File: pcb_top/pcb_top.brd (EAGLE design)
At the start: 32 x 37.3 mm, 6 parts, among them X1 FH12-14S-0.5SH

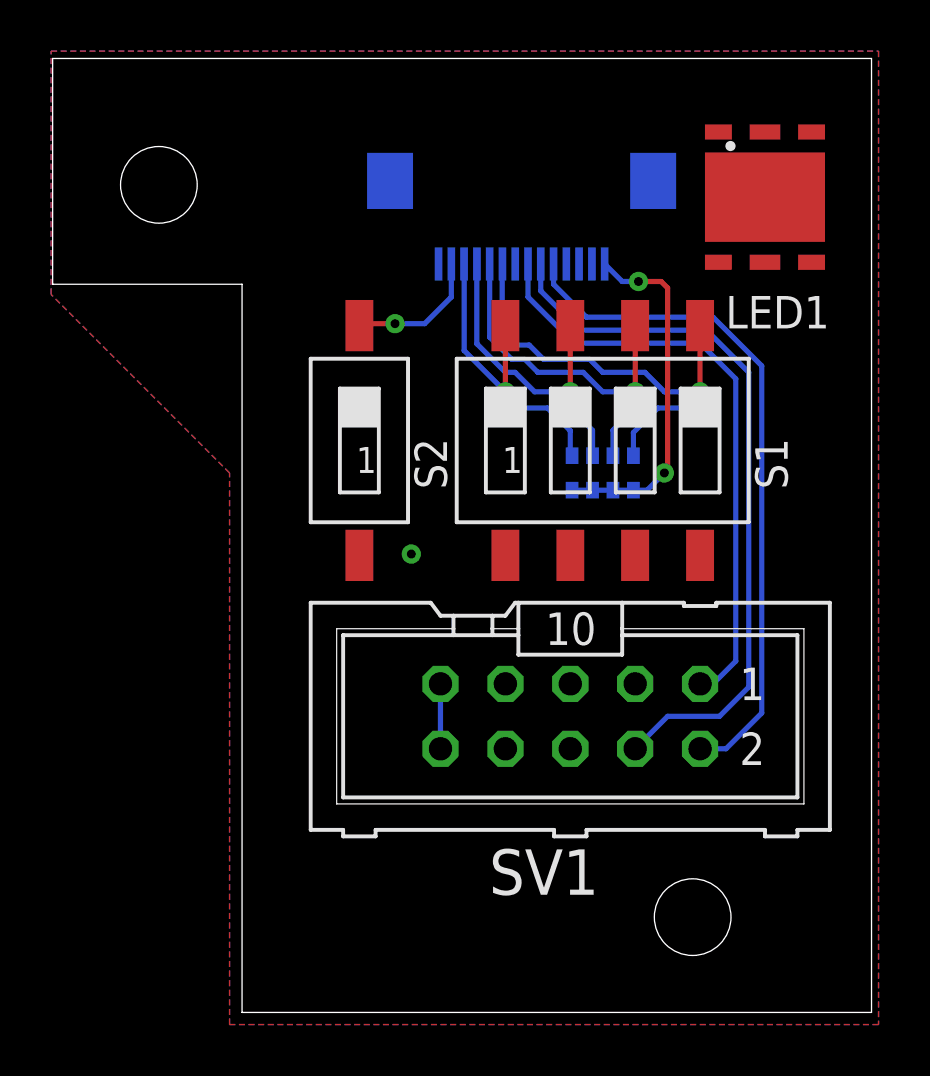
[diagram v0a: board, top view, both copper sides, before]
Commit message: finished v1.0
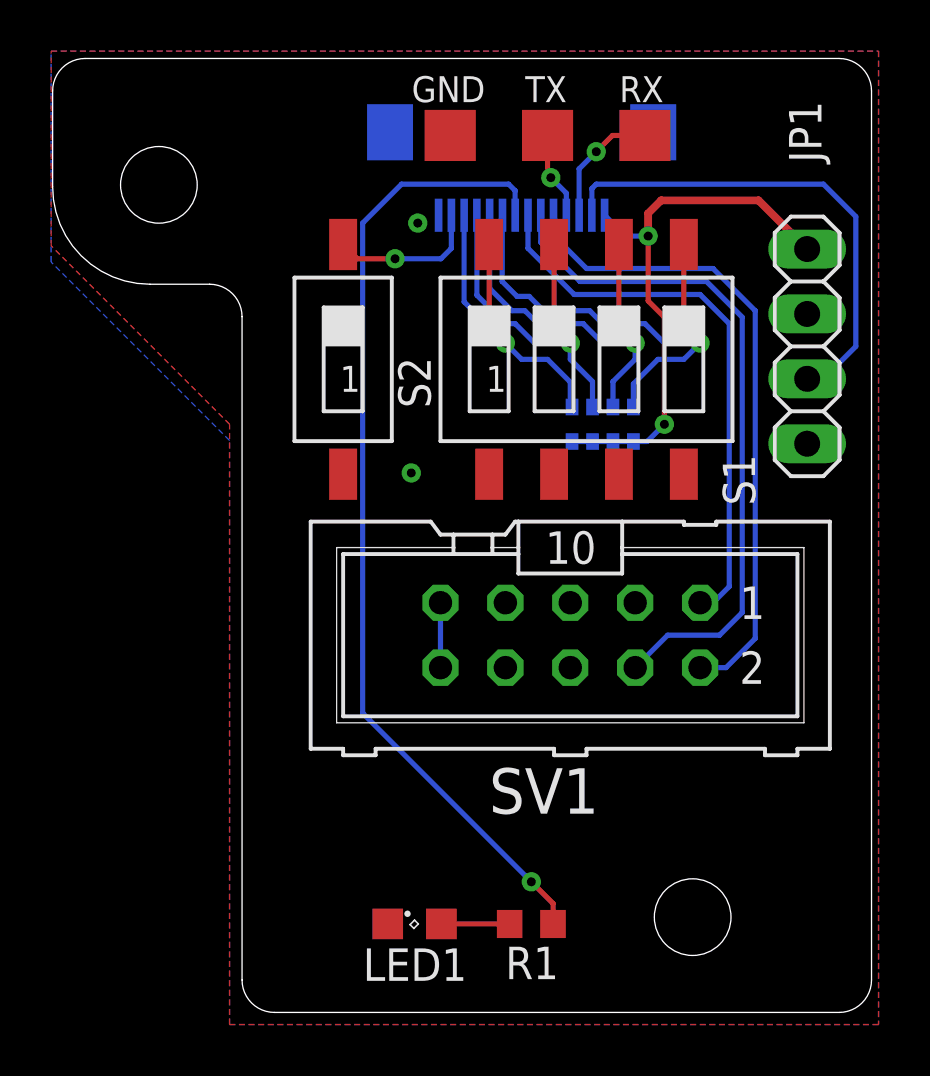
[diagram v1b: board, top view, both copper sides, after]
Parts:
- added GND, RX, TX: TPTP20SQ, testpad:TP20SQ
- added JP1: (no value), pinhead:1X04
- added R1: (no value), rcl:R0603
- LED1: value F50360 -> (none); device led:F50360 -> led:SML0805
- moved LED1 31.6 mm to (-17.9, 3.43), turned to 0 degrees
- moved S1 3.24 mm to (-11.2, 25.5)
- moved S2 3.24 mm to (-20.7, 25.5)
- moved SV1 3.17 mm to (-11.8, 14.7)
- moved X1 1.91 mm to (-13.7, 34.4)
- moved RN1 1.90 mm to (-10.5, 23.0)
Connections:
- new net N$1: LED1.A, R1.1
- net 3,3V: now also JP1.1
- net GND: now also GND.TP, JP1.2, LED1.C
- net LED: now also R1.2
- net RX: now also RX.TP
- net STARTER: now also JP1.3
- net TX: now also TX.TP
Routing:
- net LED: track 0.00 -> 38.2 mm, vias 0 -> 1
- net STARTER: track 0.00 -> 19.5 mm
- net 3,3V: track 14.0 -> 21.7 mm
- net RX: track 0.00 -> 4.93 mm, vias 0 -> 1
- net TX: track 0.00 -> 3.43 mm, vias 0 -> 1
- net N$1: track 0.00 -> 2.67 mm
- net SW4: track 18.1 -> 19.6 mm
- net SW3: track 14.9 -> 16.4 mm
- net SW2: track 13.7 -> 15.2 mm
- net SW1: track 12.4 -> 14.0 mm
- net SWDIO: track 28.3 -> 26.8 mm
- net SWCLK: track 26.8 -> 25.4 mm
- net RST: track 23.6 -> 22.1 mm
- net ROBOT_ON: track 5.36 -> 5.93 mm
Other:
- outline, holes or cut-outs redrawn
- board text added: "Miras V1.0 minisumo Dominik Pluta Kamil Winnicki"

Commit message: minor changes
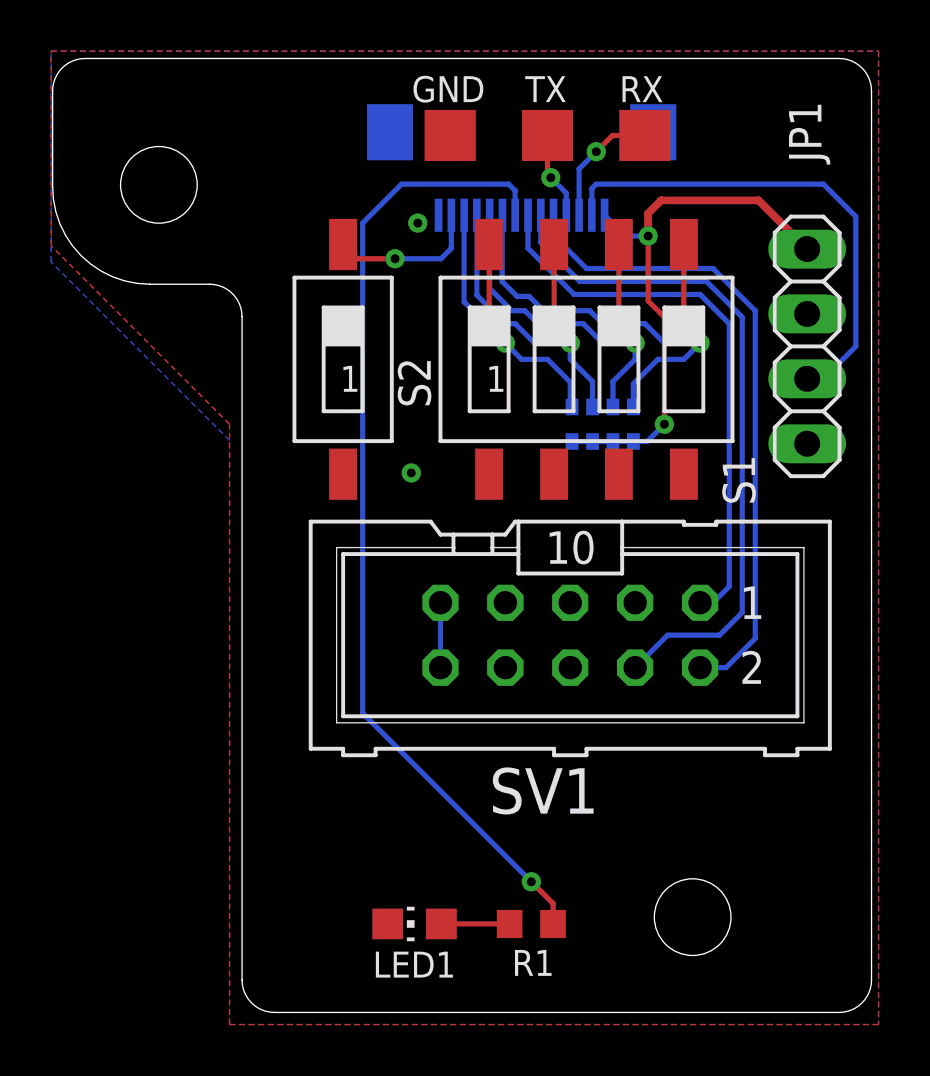
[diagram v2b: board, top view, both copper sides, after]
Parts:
- LED1: device led:SML0805 -> led:CHIP-LED0805
- turned LED1 to 90 degrees
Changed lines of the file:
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@@
 <attribute name="POPULARITY" value="9" x="-20.701" y="25.527" size="1.778" layer="27" display="off"/>
 </element>
-<element name="LED1" library="led" library_urn="urn:adsk.eagle:library:259" package="SML0805" package3d_urn="urn:adsk.eagle:package:15830/1" value="" x="-17.907" y="3.429" smashed="yes">
-<attribute name="NAME" x="-19.924" y="1.203" size="1.27" layer="25"/>
-<attribute name="POPULARITY" value="17" x="-17.907" y="3.429" size="1.778" layer="27" display="off"/>
-<attribute name="VALUE" x="-23.077" y="6.004" size="1.27" layer="27" rot="R270"/>
+<element name="LED1" library="led" library_urn="urn:adsk.eagle:library:259" package="CHIP-LED0805" package3d_urn="urn:adsk.eagle:package:15818/2" value="" x="-17.907" y="3.429" smashed="yes" rot="R90">
+<attribute name="NAME" x="-19.543" y="1.33" size="1.016" layer="25"/>
+<attribute name="POPULARITY" value="68" x="-17.907" y="3.429" size="1.778" layer="27" rot="R90" display="off"/>
+<attribute name="VALUE" x="-20.482" y="-1.741" size="1.27" layer="27"/>
 </element>
 <element name="X1" library="con-hirose" library_urn="urn:adsk.eagle:library:152" package="FH12-14S-0.5SH" package3d_urn="urn:adsk.eagle:package:7327/1" override_package3d_urn="urn:adsk.eagle:package:39279061/2" override_package_urn="urn:adsk.eagle:footprint:7251/1" value="FH12-14S-0.5SH" x="-13.716" y="34.417" smashed="yes" rot="MR180">
@@
 </element>
 <element name="R1" library="rcl" library_urn="urn:adsk.eagle:library:334" package="R0603" package3d_urn="urn:adsk.eagle:package:23555/3" value="" x="-13.335" y="3.429" smashed="yes">
-<attribute name="NAME" x="-14.351" y="1.27" size="1.27" layer="25"/>
+<attribute name="NAME" x="-14.097" y="1.397" size="1.016" layer="25"/>
 <attribute name="POPULARITY" value="70" x="-13.335" y="3.429" size="1.778" layer="27" display="off"/>
 <attribute name="SPICEPREFIX" value="R" x="-13.335" y="3.429" size="1.778" layer="27" display="off"/>
@@
 <contactref element="SV1" pad="6"/>
 <contactref element="LED1" pad="C"/>
-<contactref element="LED1" pad="C"/>
 <contactref element="JP1" pad="2"/>
 <contactref element="GND" pad="TP"/>
@@
 <contactref element="RN1" pad="7"/>
 <contactref element="RN1" pad="8"/>
-<wire x1="-9.341" y1="22.312" x2="-11.741" y2="22.312" width="0.2032" layer="16"/>
+<wire x1="-10.141" y1="22.312" x2="-10.941" y2="22.312" width="0.2032" layer="16"/>
+<wire x1="-11.43" y1="22.312" x2="-11.741" y2="22.312" width="0.2032" layer="16"/>
 <wire x1="-9.341" y1="22.312" x2="-8.802946875" y2="22.312" width="0.2032" layer="16"/>
 <wire x1="-8.802946875" y1="22.312" x2="-8.128" y2="22.987" width="0.2032" layer="16"/>
@@
 <wire x1="-8.763" y1="31.242" x2="-8.763" y2="30.353" width="0.3048" layer="1"/>
 <wire x1="-4.445" y1="31.75" x2="-8.255" y2="31.75" width="0.3048" layer="1"/>
-<wire x1="-10.941" y1="22.312" x2="-10.141" y2="22.312" width="0" layer="19" extent="16-16"/>
-<wire x1="-9.341" y1="22.312" x2="-10.141" y2="22.312" width="0" layer="19" extent="16-16"/>
+<wire x1="-10.141" y1="22.312" x2="-9.341" y2="22.312" width="0.2032" layer="16"/>
+<wire x1="-10.941" y1="22.312" x2="-11.43" y2="22.312" width="0.2032" layer="16"/>
 </signal>
 <signal name="5V_ST-LINK">
